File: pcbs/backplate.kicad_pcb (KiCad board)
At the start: 2 copper layers, 133.8 x 91.7 mm, 5 parts

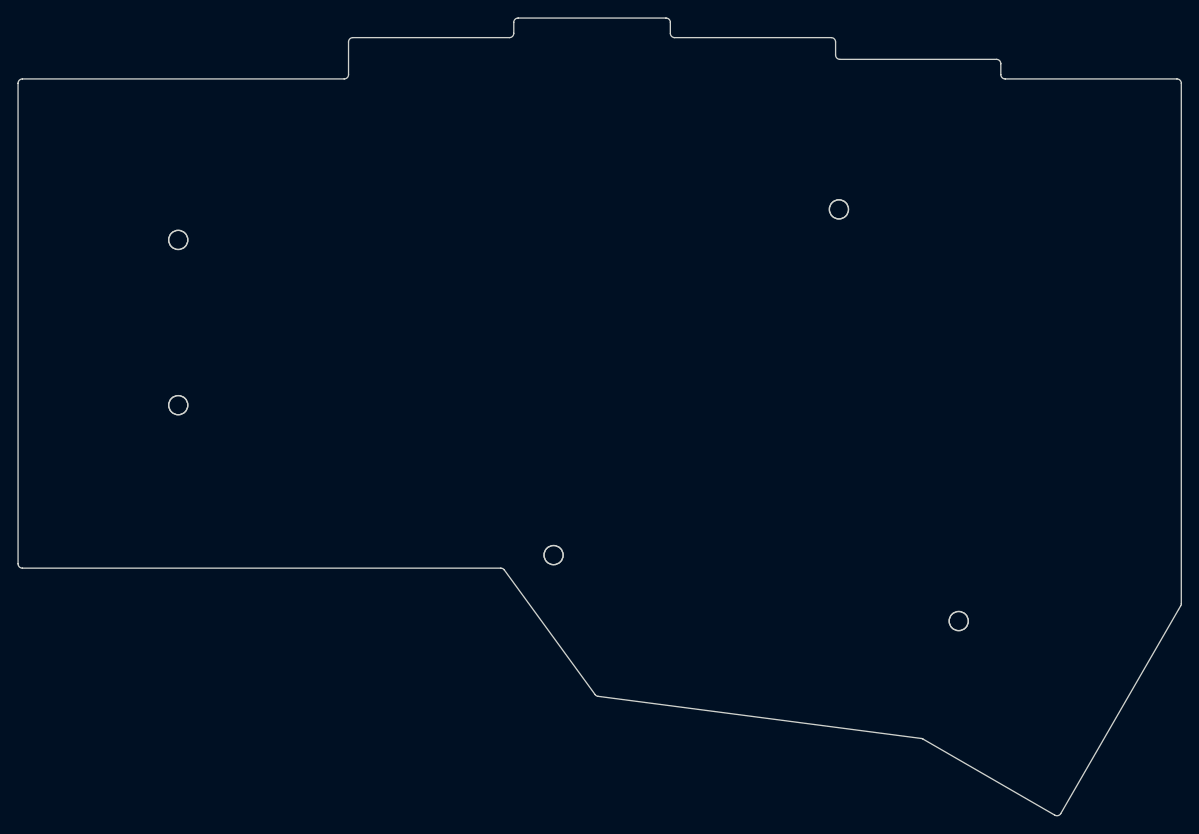
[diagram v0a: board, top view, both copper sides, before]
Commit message: build: regenerate outlines and PCBs with Ergogen snapshot
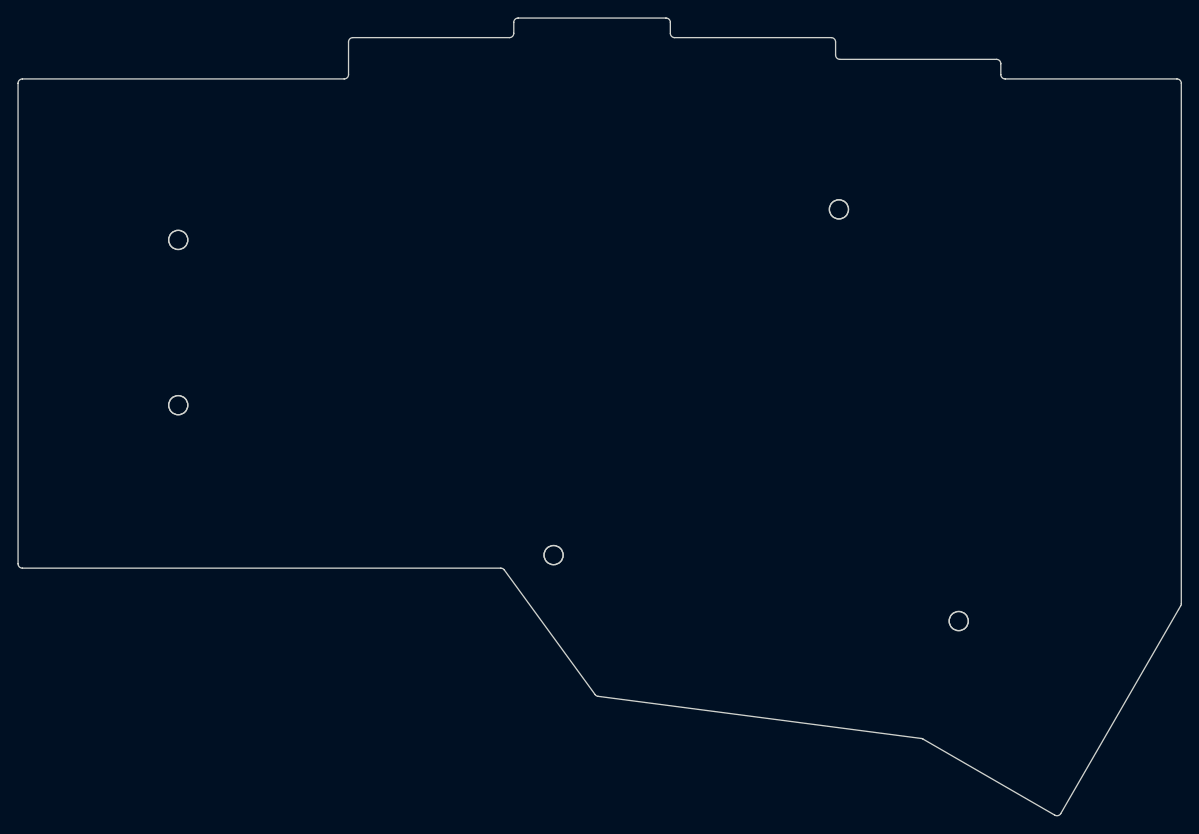
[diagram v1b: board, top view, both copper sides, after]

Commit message: build: regenerate PCBs, images, and gerbers
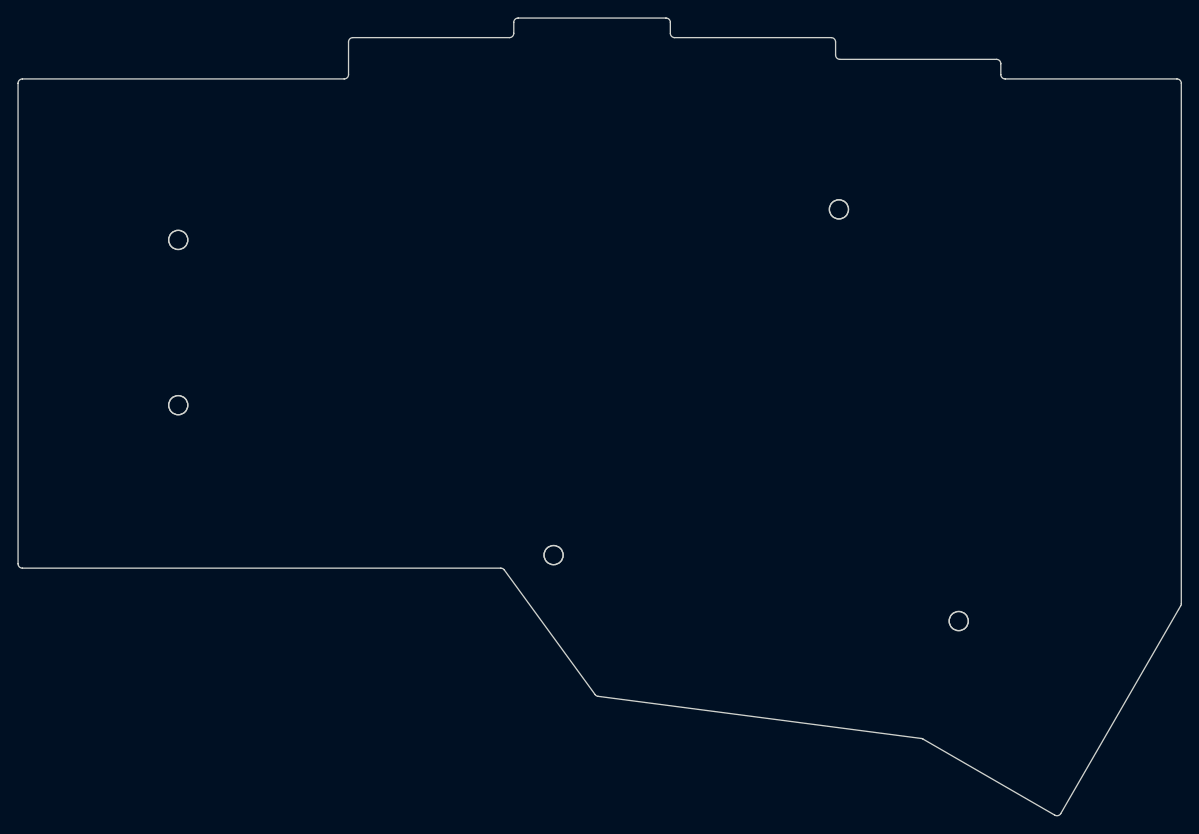
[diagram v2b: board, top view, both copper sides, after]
